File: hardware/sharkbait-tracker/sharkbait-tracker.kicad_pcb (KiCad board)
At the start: 2 copper layers, 3 parts, among them U1 LLCC68, U2 STM32L031G6Ux, Y1 32MHz

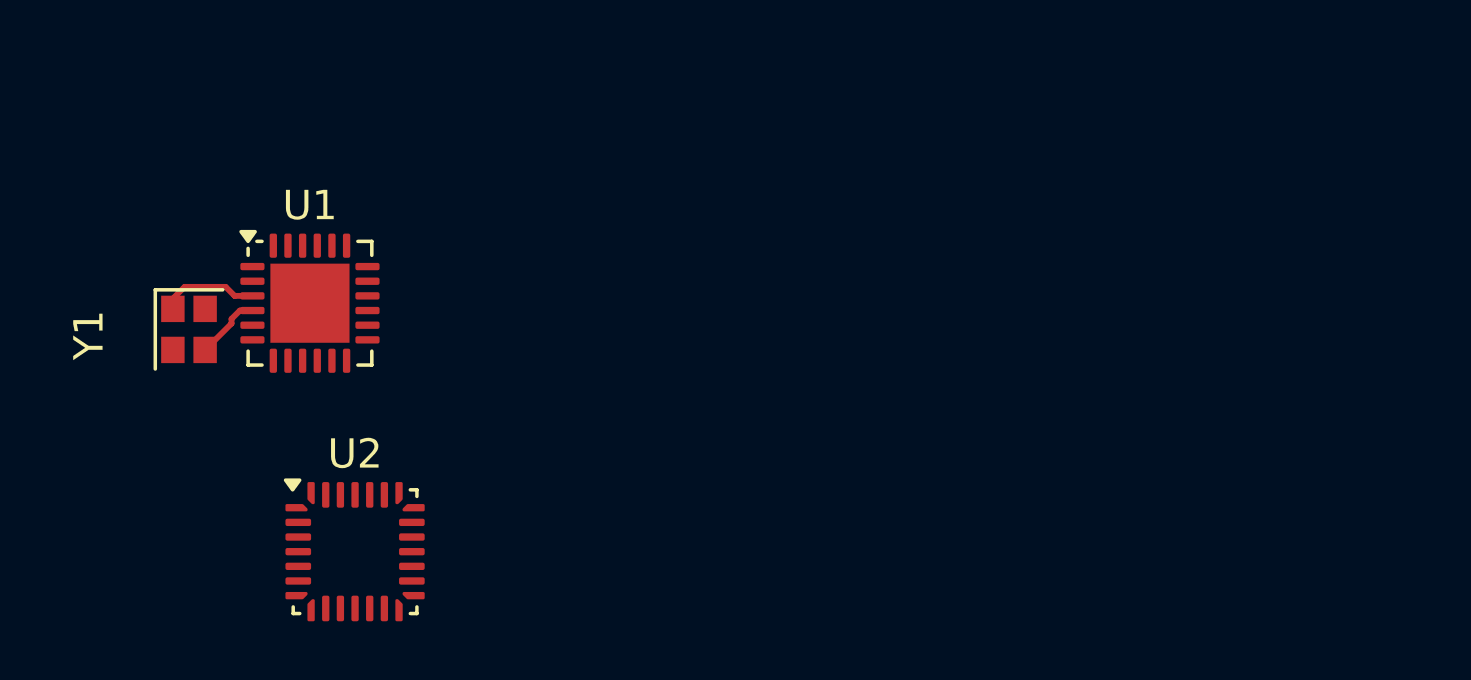
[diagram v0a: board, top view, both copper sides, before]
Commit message: Most of the layout done, but might break things
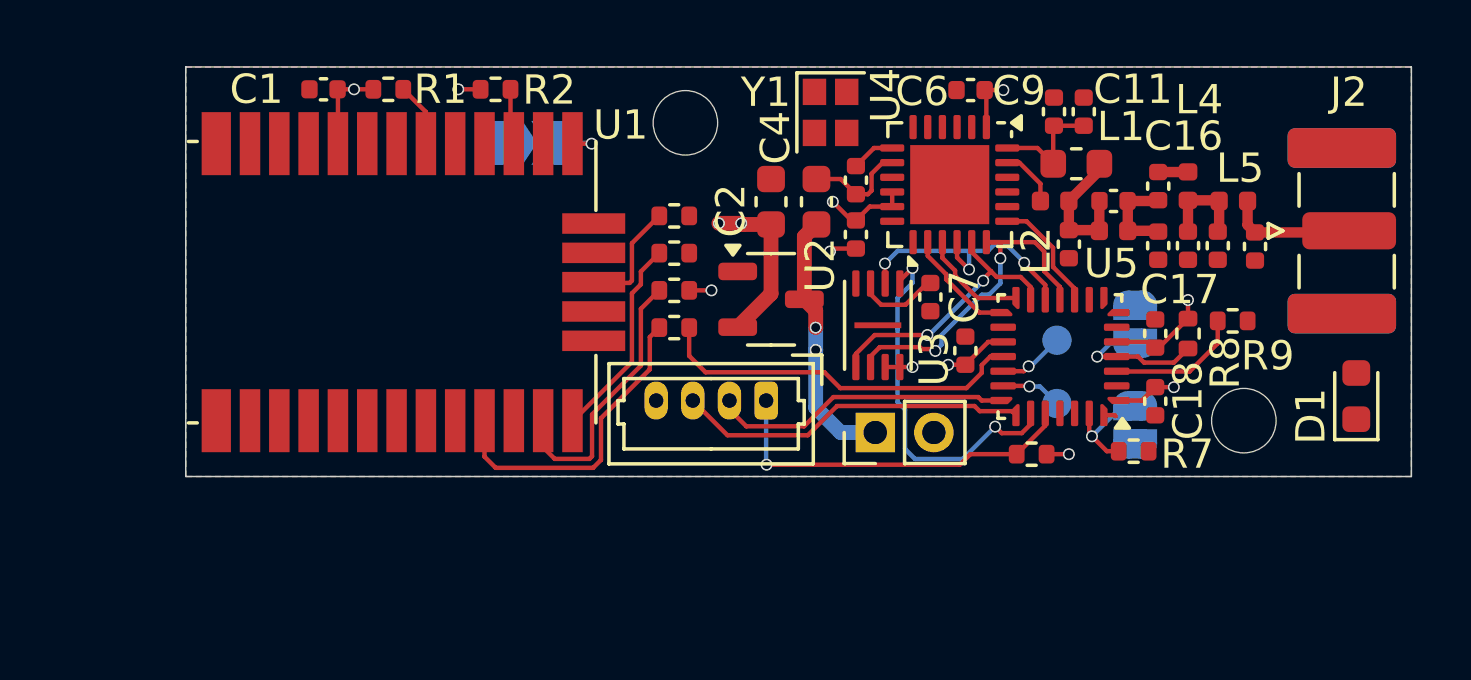
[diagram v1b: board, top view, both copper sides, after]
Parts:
- added BT1: LiPo, Connector_PinHeader_2.00mm:PinHeader_1x02_P2.00mm_Vertical, F.Cu at (126.5, 83.8)
- added C1: 0.1uF, Capacitor_SMD:C_0402_1005Metric, F.Cu at (107.7, 72.1)
- added C10: 6.8p, Capacitor_SMD:C_0402_1005Metric, F.Cu at (133.1, 77.4)
- added C11: 0.1uF, Capacitor_SMD:C_0402_1005Metric, F.Cu at (133.6, 72.9)
- added C12: 6.8p, Capacitor_SMD:C_0402_1005Metric, F.Cu at (134.6, 75.9)
- added C13: 4.7p, Capacitor_SMD:C_0402_1005Metric, F.Cu at (136.1, 77.5)
- added C14: 0, Capacitor_SMD:C_0402_1005Metric, F.Cu at (138.2, 77.5)
- added C15: 3.3p, Capacitor_SMD:C_0402_1005Metric, F.Cu at (137.2, 77.5)
- added C16: 68p, Capacitor_SMD:C_0402_1005Metric, F.Cu at (136.1, 75.4)
- added C17: 0.1uF, Capacitor_SMD:C_0402_1005Metric, F.Cu at (136.0, 80.5)
- added C18: 0.1uF, Capacitor_SMD:C_0402_1005Metric, F.Cu at (136.0, 82.8)
- added C19: 0, Capacitor_SMD:C_0402_1005Metric, F.Cu at (139.4, 77.5)
- added C2: 10uF, Capacitor_SMD:C_0603_1608Metric, F.Cu at (122.9, 76.0)
- added C3: 1uF, Capacitor_SMD:C_0402_1005Metric, F.Cu at (125.8, 75.2)
- added C4: 10uF, Capacitor_SMD:C_0603_1608Metric, F.Cu at (124.5, 76.0)
- added C5: 0.1uF, Capacitor_SMD:C_0402_1005Metric, F.Cu at (125.8, 77.1)
- added C6: 1uF, Capacitor_SMD:C_0402_1005Metric, F.Cu at (129.7, 72.2)
- added C7: 0.1uF, Capacitor_SMD:C_0402_1005Metric, F.Cu at (128.4, 79.2)
- added C8: 0.1uF, Capacitor_SMD:C_0402_1005Metric, F.Cu at (129.6, 81.1)
- added C9: 68p, Capacitor_SMD:C_0402_1005Metric, F.Cu at (132.6, 72.9)
- added D1: RED, LED_SMD:LED_0603_1608Metric, F.Cu at (142.9, 82.6)
- added H1: MountingHole, MountingHole:MountingHole_2.2mm_M2, F.Cu at (120.0, 73.3)
- added H2: MountingHole, MountingHole:MountingHole_2.2mm_M2, F.Cu at (139.1, 83.4)
- added J1: Conn_01x04, Connector_Molex:Molex_PicoBlade_53047-0410_1x04_P1.25mm_Vertical, F.Cu at (122.8, 82.8)
- added J2: Conn_Coaxial_Small, Connector_Coaxial:SMA_Samtec_SMA-J-P-H-ST-EM1_EdgeMount, F.Cu at (142.7, 77.0)
- added JP1: RST, Jumper:SolderJumper-2_P1.3mm_Open_RoundedPad1.0x1.5mm, B.Cu at (135.4, 80.2)
- added JP2: BOOT, Jumper:SolderJumper-2_P1.3mm_Open_RoundedPad1.0x1.5mm, B.Cu at (135.4, 83.6)
- added JP3: Ublox_VCCIO, Jumper:SolderJumper-2_P1.3mm_Open_TrianglePad1.0x1.5mm, B.Cu at (114.7, 74.0)
- added L1: 68u, Inductor_SMD:L_0603_1608Metric, F.Cu at (133.3, 74.7)
- added L2: 4.7n, Inductor_SMD:L_0402_1005Metric, F.Cu at (132.6, 75.9)
- added L3: 3.9n, Inductor_SMD:L_0402_1005Metric, F.Cu at (134.6, 77.0)
- added L4: 10n, Inductor_SMD:L_0402_1005Metric, F.Cu at (137.2, 75.4)
- added L5: 0R, Inductor_SMD:L_0402_1005Metric, F.Cu at (138.7, 75.9)
- added R1: 4.7k, Resistor_SMD:R_0402_1005Metric, F.Cu at (109.9, 72.1)
- added R10: 220, Resistor_SMD:R_0402_1005Metric, F.Cu at (119.6, 76.5)
- added R11: 220, Resistor_SMD:R_0402_1005Metric, F.Cu at (119.6, 80.3)
- added R12: 4.7k, Resistor_SMD:R_0402_1005Metric, F.Cu at (131.8, 84.6)
- added R2: 4.7k, Resistor_SMD:R_0402_1005Metric, F.Cu at (113.5, 72.1)
- added R3: 220, Resistor_SMD:R_0402_1005Metric, F.Cu at (119.6, 79.0)
- added R4: 220, Resistor_SMD:R_0402_1005Metric, F.Cu at (119.6, 77.7)
- added R7: 4.7k, Resistor_SMD:R_0402_1005Metric, F.Cu at (135.3, 84.5)
- added R8: 4.7k, Resistor_SMD:R_0402_1005Metric, F.Cu at (137.2, 80.5)
- added R9: 75, Resistor_SMD:R_0402_1005Metric, F.Cu at (138.7, 80.0)
- added TP1: DBG_RX, TestPoint:TestPoint_Pad_D1.0mm, B.Cu at (132.7, 82.9)
- added TP2: DBG_TX, TestPoint:TestPoint_Pad_D1.0mm, B.Cu at (132.7, 80.7)
- added U2: XC6206PxxxMR, Package_TO_SOT_SMD:SOT-23-3, F.Cu at (122.9, 79.3)
- added U3: XT25F32FDTIGT, Package_SON:Winbond_USON-8-1EP_3x2mm_P0.5mm_EP0.2x1.6mm, F.Cu at (126.6, 80.2)
- added U4: LLCC68, Package_DFN_QFN:QFN-24-1EP_4x4mm_P0.5mm_EP2.7x2.7mm, F.Cu at (129.0, 75.4)
- U1: value LLCC68 -> Quectel_L96; footprint Package_DFN_QFN:QFN-24-1EP_4x4mm_P0.5mm_EP2.7x2.7mm -> RF_Module_Custom:CAM-M8_QuectelL96
- moved U5 24.9 mm to (132.8, 81.3), turned to 180 degrees
- moved Y1 23.1 mm to (125.0, 72.9)
- moved U1 4.31 mm to (103.0, 78.7), turned to 90 degrees
- renumbered U2 to U5
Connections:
- U1 pad 1: +3.3V -> /UBLOX_VCCIO
- U1 pad 10: +3.3V -> GND
- U1 pad 11: +3.3V -> GND
- U1 pad 12: unconnected-(U1-DIO2-Pad12) -> GND
- U1 pad 13: unconnected-(U1-DIO1-Pad13) -> GND
- U1 pad 14: unconnected-(U1-BUSY-Pad14) -> GND
- U1 pad 15: unconnected-(U1-NRESET-Pad15) -> GND
- U1 pad 16: unconnected-(U1-MISO-Pad16) -> Net-(U1-RF_IN)
- U1 pad 17: unconnected-(U1-MOSI-Pad17) -> Net-(U1-RF_IN)
- U1 pad 18: unconnected-(U1-SCK-Pad18) -> GND
- U1 pad 19: unconnected-(U1-NSS-Pad19) -> GND
- U1 pad 2: GND -> unconnected-(U1-3D_FIX-Pad2)
- U1 pad 20: GND -> unconnected-(U1-JAM_IND-Pad20)
- U1 pad 21: Net-(U1-RFI_N) -> GND
- U1 pad 22: Net-(U1-RFI_N) -> GND
- U1 pad 23: unconnected-(U1-RFO-Pad23) -> /R_nRST
- U1 pad 25: GND -> /GPS_TX
- U1 pad 3: /RF_XTA -> /SDA_NC
- U1 pad 4: /RF_XTB -> GND
- U1 pad 6: unconnected-(U1-DIO3-Pad6) -> /SCL_NC
- U1 pad 8: GND -> +3.3V
- U1 pad 9: unconnected-(U1-DCC_SW-Pad9) -> +3.3V
- U5 pad 10: unconnected-(U2-PA4-Pad10) -> /RF_CS
- U5 pad 11: unconnected-(U2-PA5-Pad11) -> /SCK
- U5 pad 12: unconnected-(U2-PA6-Pad12) -> /MISO
- U5 pad 13: unconnected-(U2-PA7-Pad13) -> /MOSI
- U5 pad 14: unconnected-(U2-PB0-Pad14) -> /RF_nRST
- U5 pad 15: unconnected-(U2-PB1-Pad15) -> /RF_BUSY
- U5 pad 18: unconnected-(U2-PA8-Pad18) -> /GPS_nRST
- U5 pad 19: unconnected-(U2-PA9-Pad19) -> /DBG_TX
- U5 pad 20: unconnected-(U2-PA10-Pad20) -> /DBG_RX
- U5 pad 21: unconnected-(U2-PA13-Pad21) -> /SWDIO
- U5 pad 22: unconnected-(U2-PA14-Pad22) -> /SWCLK
- U5 pad 23: unconnected-(U2-PA15-Pad23) -> /FLASH_CS
- U5 pad 24: unconnected-(U2-PB3-Pad24) -> /OWI
- U5 pad 27: unconnected-(U2-BOOT0-Pad27) -> /BOOT
- U5 pad 3: unconnected-(U2-PC15-Pad3) -> /LED
- U5 pad 4: unconnected-(U2-NRST-Pad4) -> /NRST
- U5 pad 6: unconnected-(U2-PA0-Pad6) -> /GPS_1PPS
- U5 pad 8: unconnected-(U2-PA2-Pad8) -> /TX
- U5 pad 9: unconnected-(U2-PA3-Pad9) -> /RX
- Y1 pad 1: /RF_XTA -> /RF Transmitter/RF_XTA
- Y1 pad 3: /RF_XTB -> /RF Transmitter/RF_XTB
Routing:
- net +3.3V: track 0.00 -> 26.9 mm, vias 0 -> 11
- net /GPS_nRST: track 0.00 -> 12.7 mm
- net /OWI: track 0.00 -> 12.7 mm, vias 0 -> 1
- net /FLASH_CS: track 0.00 -> 12.7 mm, vias 0 -> 2
- net /SWCLK: track 0.00 -> 12.1 mm
- net /SCK: track 0.00 -> 12.0 mm, vias 0 -> 2
- net /R_nRST: track 0.00 -> 10.8 mm
- net /SWDIO: track 0.00 -> 10.3 mm
- net /MOSI: track 0.00 -> 9.53 mm, vias 0 -> 2
- net /GPS_TX: track 0.00 -> 9.36 mm
- net /MISO: track 0.00 -> 9.29 mm, vias 0 -> 3
- net +BATT: track 0.00 -> 8.96 mm, vias 0 -> 2
- net /GPS_RX: track 0.00 -> 6.97 mm
- net GND: track 0.00 -> 4.93 mm, vias 0 -> 1
- net /NRST: track 0.00 -> 4.87 mm, vias 0 -> 1
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- added copper zone on B.Cu, net +3.3V
- added copper zone on F.Cu, net GND
- added copper zone on In1.Cu, net GND
- added copper zone on In2.Cu, net GND
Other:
- board outline added: 41.8 x 14 mm
- copper layers 2 -> 4
- board text added: "RST BOOT"
- board text added: "TX RX"
